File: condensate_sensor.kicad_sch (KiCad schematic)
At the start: 3 parts

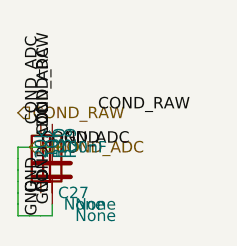
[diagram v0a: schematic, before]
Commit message: fix writer
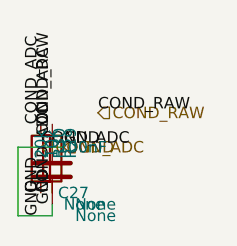
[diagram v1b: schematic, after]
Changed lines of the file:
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@@
 		(instances
 			(project "Untitled"
-				(path "/a59e5e4e-0756-472a-ad31-66ebbca15e78"
+				(path "/7f9dfed3-5cce-4152-9ab6-c9be91e704d9"
 					(reference "C27")
 					(unit 1)
@@
 		(instances
 			(project "Untitled"
-				(path "/a59e5e4e-0756-472a-ad31-66ebbca15e78"
+				(path "/7f9dfed3-5cce-4152-9ab6-c9be91e704d9"
 					(reference "R29")
 					(unit 1)
@@
 		(instances
 			(project "Untitled"
-				(path "/a59e5e4e-0756-472a-ad31-66ebbca15e78"
+				(path "/7f9dfed3-5cce-4152-9ab6-c9be91e704d9"
 					(reference "R30")
 					(unit 1)
@@
 	(wire
 		(pts
-			(xy 16.51 24.13) (xy 15.24 24.13)
-		)
-		(stroke
-			(width 0)
-			(type default)
-		)
-	)
-	(wire
-		(pts
-			(xy 15.24 24.13) (xy 13.97 24.13)
-		)
-		(stroke
-			(width 0)
-			(type default)
-		)
-	)
-	(wire
-		(pts
-			(xy 13.97 24.13) (xy 12.7 24.13)
-		)
-		(stroke
-			(width 0)
-			(type default)
-		)
-	)
-	(wire
-		(pts
-			(xy 12.7 24.13) (xy 12.7 22.86)
-		)
-		(stroke
-			(width 0)
-			(type default)
-		)
-	)
-	(wire
-		(pts
-			(xy 12.7 22.86) (xy 12.7 21.59)
-		)
-		(stroke
-			(width 0)
-			(type default)
-		)
-	)
-	(wire
-		(pts
-			(xy 12.7 21.59) (xy 12.7 20.32)
-		)
-		(stroke
-			(width 0)
-			(type default)
-		)
-	)
-	(wire
-		(pts
-			(xy 12.7 20.32) (xy 12.7 19.05)
-		)
-		(stroke
-			(width 0)
-			(type default)
-		)
-	)
-	(wire
-		(pts
-			(xy 12.7 19.05) (xy 12.7 17.78)
-		)
-		(stroke
-			(width 0)
-			(type default)
-		)
-	)
-	(wire
-		(pts
-			(xy 12.7 17.78) (xy 12.7 16.51)
+			(xy 16.51 24.13) (xy 12.7 24.13)
+		)
+		(stroke
+			(width 0)
+			(type default)
+		)
+	)
+	(wire
+		(pts
+			(xy 12.7 24.13) (xy 12.7 16.51)
 		)
 		(stroke
@@
 	(hierarchical_label "GND"
 		(shape input)
-		(at 13.97 16.51 180)
+		(at 17.78 16.51 180)
 		(effects
 			(font
@@
 	(hierarchical_label "COND_RAW"
 		(shape input)
-		(at 12.7 12.7 180)
-		(effects
-			(font
+		(at 21.59 12.7 180)
+		(effects
+			(font
